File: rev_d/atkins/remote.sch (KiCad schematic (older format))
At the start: 67 parts, among them J1 Conn_01x05_Female, J10 Conn_01x03_Female, J2 Conn_01x07_Female, J3 Micro_SD_Card, J4 U_FL-R-SMT-1_10_, J5 Conn_01x05_Female, J6 USB_B_Micro, J7 Conn_01x04_Female, J8 Conn_01x04_Male, J9 SCD30, Q1 Q_NPN_BEC, Q2 Q_NPN_BEC, Q3 Q_PMOS_GSD - DMG3415U, SW2 SPST_TACT-KMR2, SW3 SPST_TACT-KMR2, SW4 SW_Push, SW5 SW_Push, U1 RFM95HW, U2 ESP32-WROOM, U3 MCP73831_2, U4 CP2104, U5 AP2112K-3.3, U6 AP2112K-3.3, U7 AP2112K-3.3, X1 CON_JST_PH_2PIN, X2 CON_JST_PH_2PIN, u18 BMP388

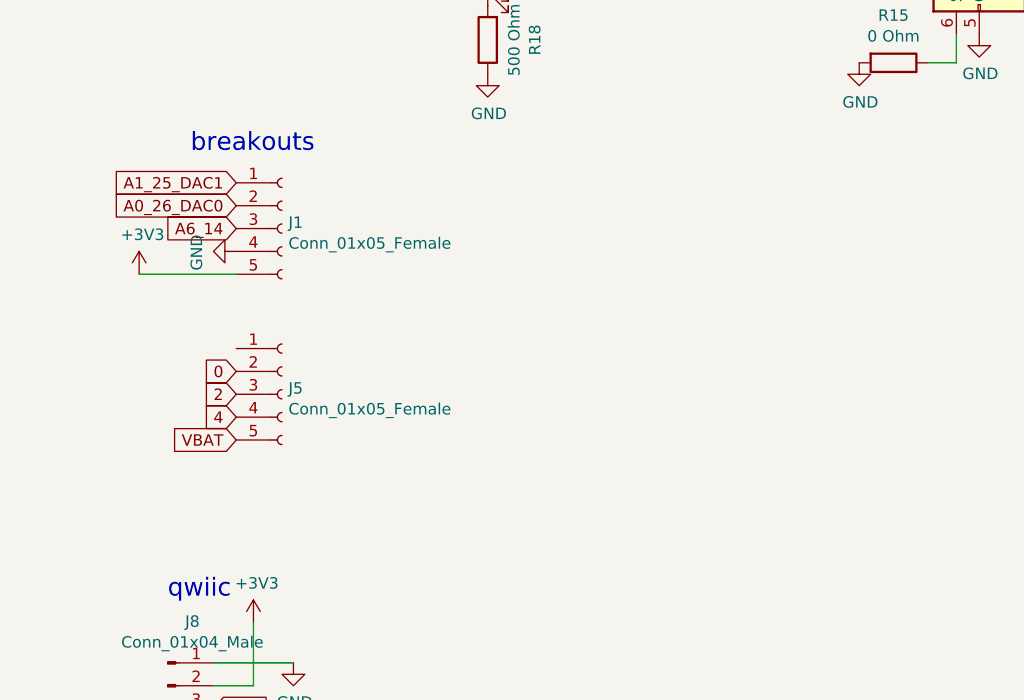
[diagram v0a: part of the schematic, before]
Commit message: update
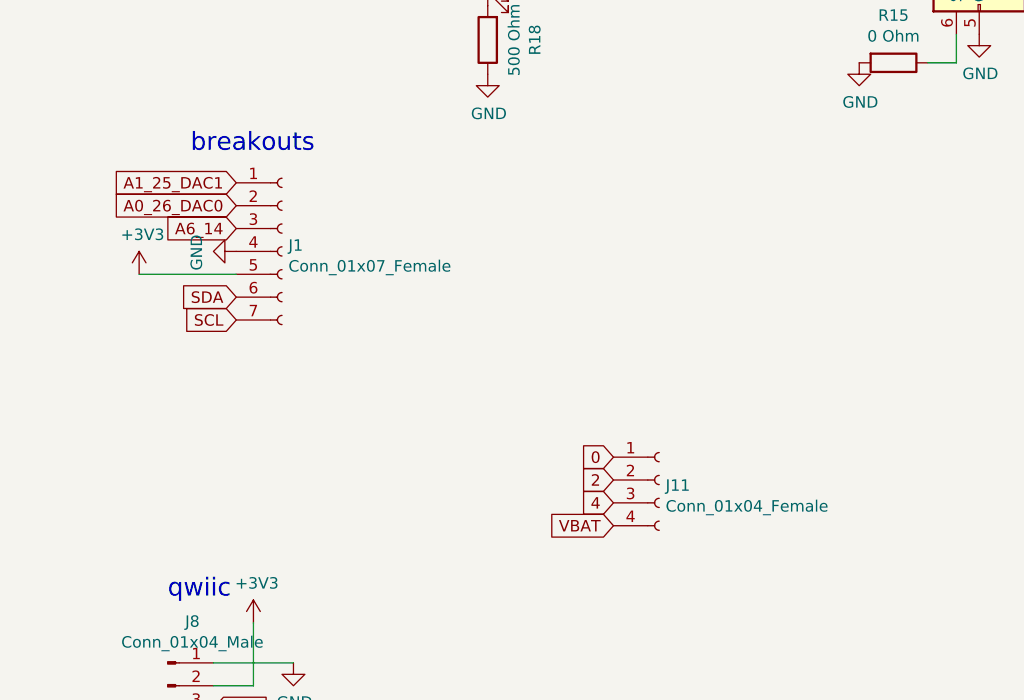
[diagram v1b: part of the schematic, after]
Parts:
- removed J1, J5: Conn_01x05_Female, Connector_PinSocket_2.54mm:PinSocket_1x05_P2.54mm_Vertical, symbol Connector:Conn_01x05_Female
- added J1: Conn_01x07_Female, Connector_PinSocket_2.54mm:PinSocket_1x07_P2.54mm_Vertical, symbol Connector:Conn_01x07_Female
- added J11: Conn_01x04_Female, Connector_PinSocket_2.54mm:PinSocket_1x04_P2.54mm_Vertical, symbol Connector:Conn_01x04_Female
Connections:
- net +3V3: now also J1.5 (Pin_5)
- net 0: now also J11.1 (Pin_1)
- net 2: now also J11.2 (Pin_2)
- net 4: now also J11.3 (Pin_3)
- net A0_26_DAC0: now also J1.2 (Pin_2)
- net A1_25_DAC1: now also J1.1 (Pin_1)
- net A6_14: now also J1.3 (Pin_3)
- net GND: now also J1.4 (Pin_4)
- net SCL: now also J1.7 (Pin_7)
- net SDA: now also J1.6 (Pin_6)
- net VBAT: now also J11.4 (Pin_4)
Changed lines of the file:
@@
 Text GLabel 13300 3700 3    50   Input ~ 0
 A8_15
-Text GLabel 13300 6000 0    50   Input ~ 0
+Text GLabel 14950 6375 0    50   Input ~ 0
 4
-Text GLabel 13300 5900 0    50   Input ~ 0
+Text GLabel 14950 6275 0    50   Input ~ 0
 2
-Text GLabel 13300 5800 0    50   Input ~ 0
+Text GLabel 14950 6175 0    50   Input ~ 0
 0
 Text GLabel 10150 1775 0    50   Input ~ 0
@@
 Text GLabel 14400 3900 0    50   Input ~ 0
 A11_12
-$Comp
-L Connector:Conn_01x05_Female J5
-U 1 1 600DC2A3
-P 13500 5900
-F 0 "J5" H 13528 5926 50  0000 L CNN
-F 1 "Conn_01x05_Female" H 13528 5835 50  0000 L CNN
-F 2 "Connector_PinSocket_2.54mm:PinSocket_1x05_P2.54mm_Vertical" H 13500 5900 50  0001 C CNN
-F 3 "~" H 13500 5900 50  0001 C CNN
-	1    13500 5900
-	1    0    0    -1
-$EndComp
-Text GLabel 13300 6100 0    50   Input ~ 0
+Text GLabel 14950 6475 0    50   Input ~ 0
 VBAT
 Text GLabel 2850 3975 2    50   Input ~ 0
@@
 Wire Wire Line
 	13300 5375 12875 5375
-$Comp
-L Connector:Conn_01x05_Female J1
-U 1 1 603068CE
-P 13500 5175
-F 0 "J1" H 13528 5201 50  0000 L CNN
-F 1 "Conn_01x05_Female" H 13528 5110 50  0000 L CNN
-F 2 "Connector_PinSocket_2.54mm:PinSocket_1x05_P2.54mm_Vertical" H 13500 5175 50  0001 C CNN
-F 3 "~" H 13500 5175 50  0001 C CNN
-	1    13500 5175
-	1    0    0    -1
-$EndComp
 Text Notes 2650 1275 0    79   ~ 0
 battery charging
@@
 	1    0    0    -1
 $EndComp
+$Comp
+L Connector:Conn_01x04_Female J11
+U 1 1 5FF2300C
+P 15150 6275
+F 0 "J11" H 15178 6251 50  0000 L CNN
+F 1 "Conn_01x04_Female" H 15178 6160 50  0000 L CNN
+F 2 "Connector_PinSocket_2.54mm:PinSocket_1x04_P2.54mm_Vertical" H 15150 6275 50  0001 C CNN
+F 3 "~" H 15150 6275 50  0001 C CNN
+	1    15150 6275
+	1    0    0    -1
+$EndComp
+$Comp
+L Connector:Conn_01x07_Female J1
+U 1 1 5FF3A551
+P 13500 5275
+F 0 "J1" H 13528 5301 50  0000 L CNN
+F 1 "Conn_01x07_Female" H 13528 5210 50  0000 L CNN
+F 2 "Connector_PinSocket_2.54mm:PinSocket_1x07_P2.54mm_Vertical" H 13500 5275 50  0001 C CNN
+F 3 "~" H 13500 5275 50  0001 C CNN
+	1    13500 5275
+	1    0    0    -1
+$EndComp
+Text GLabel 13300 5475 0    50   Input ~ 0
+SDA
+Text GLabel 13300 5575 0    50   Input ~ 0
+SCL
 $EndSCHEMATC
